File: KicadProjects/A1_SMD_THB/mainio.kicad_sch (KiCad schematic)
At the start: 6 parts, among them J3 PCF, J5 EXF, J6 THO, J7 HE, J8 BL_PROBE, J9 BL_SERVO

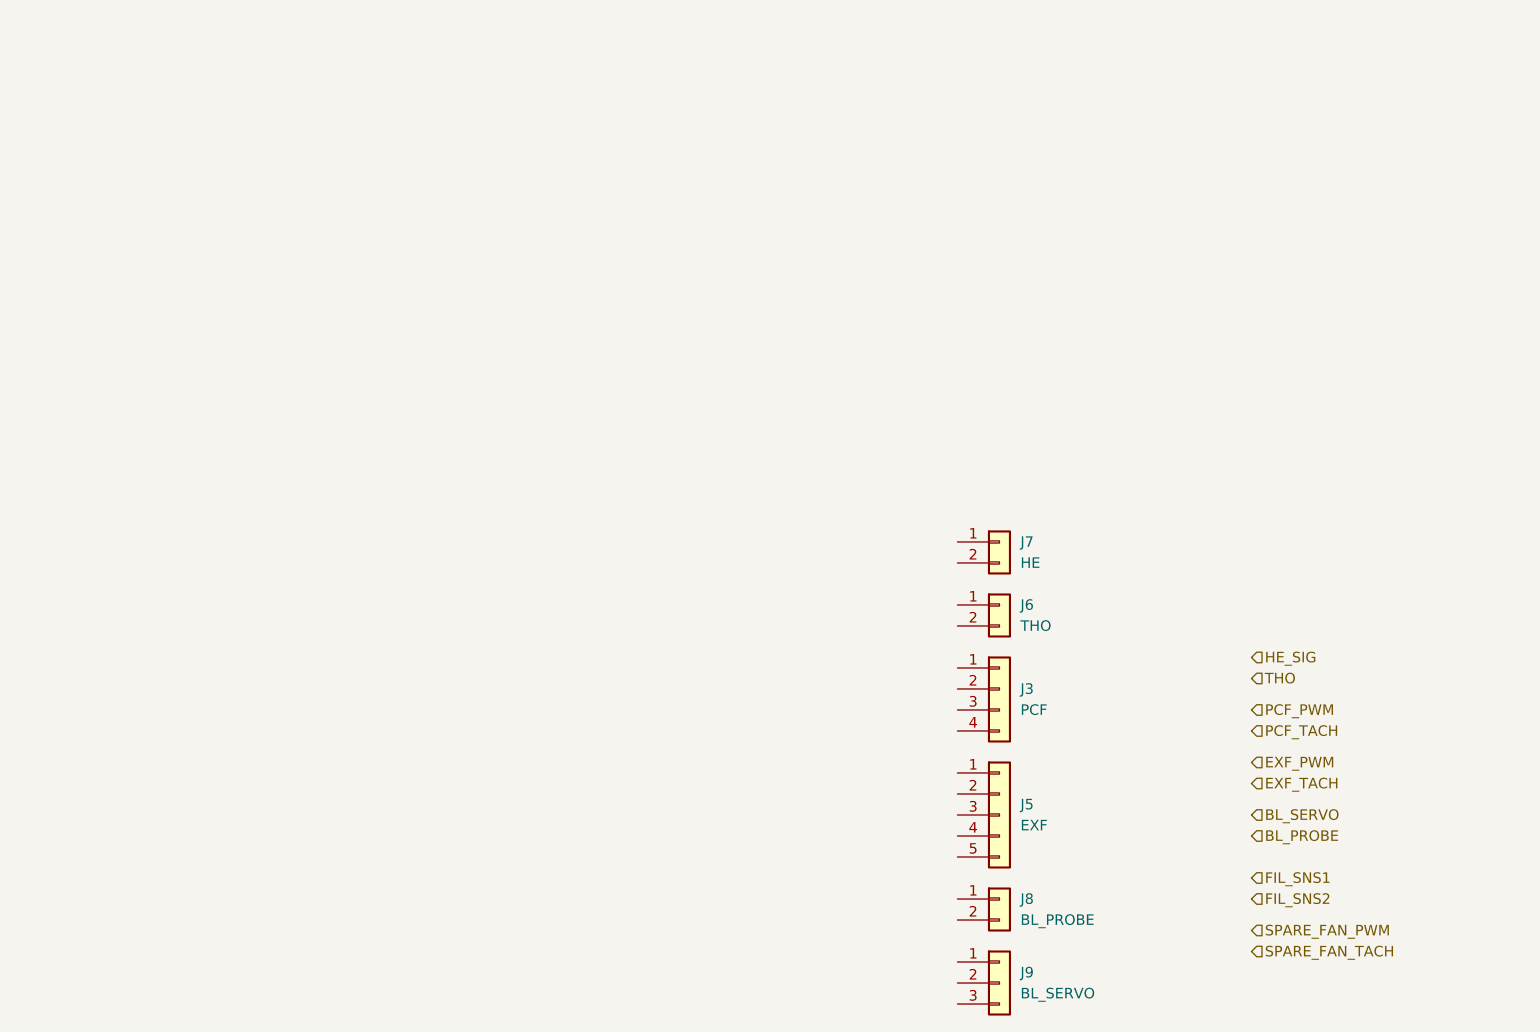
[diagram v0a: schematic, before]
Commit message: e
e
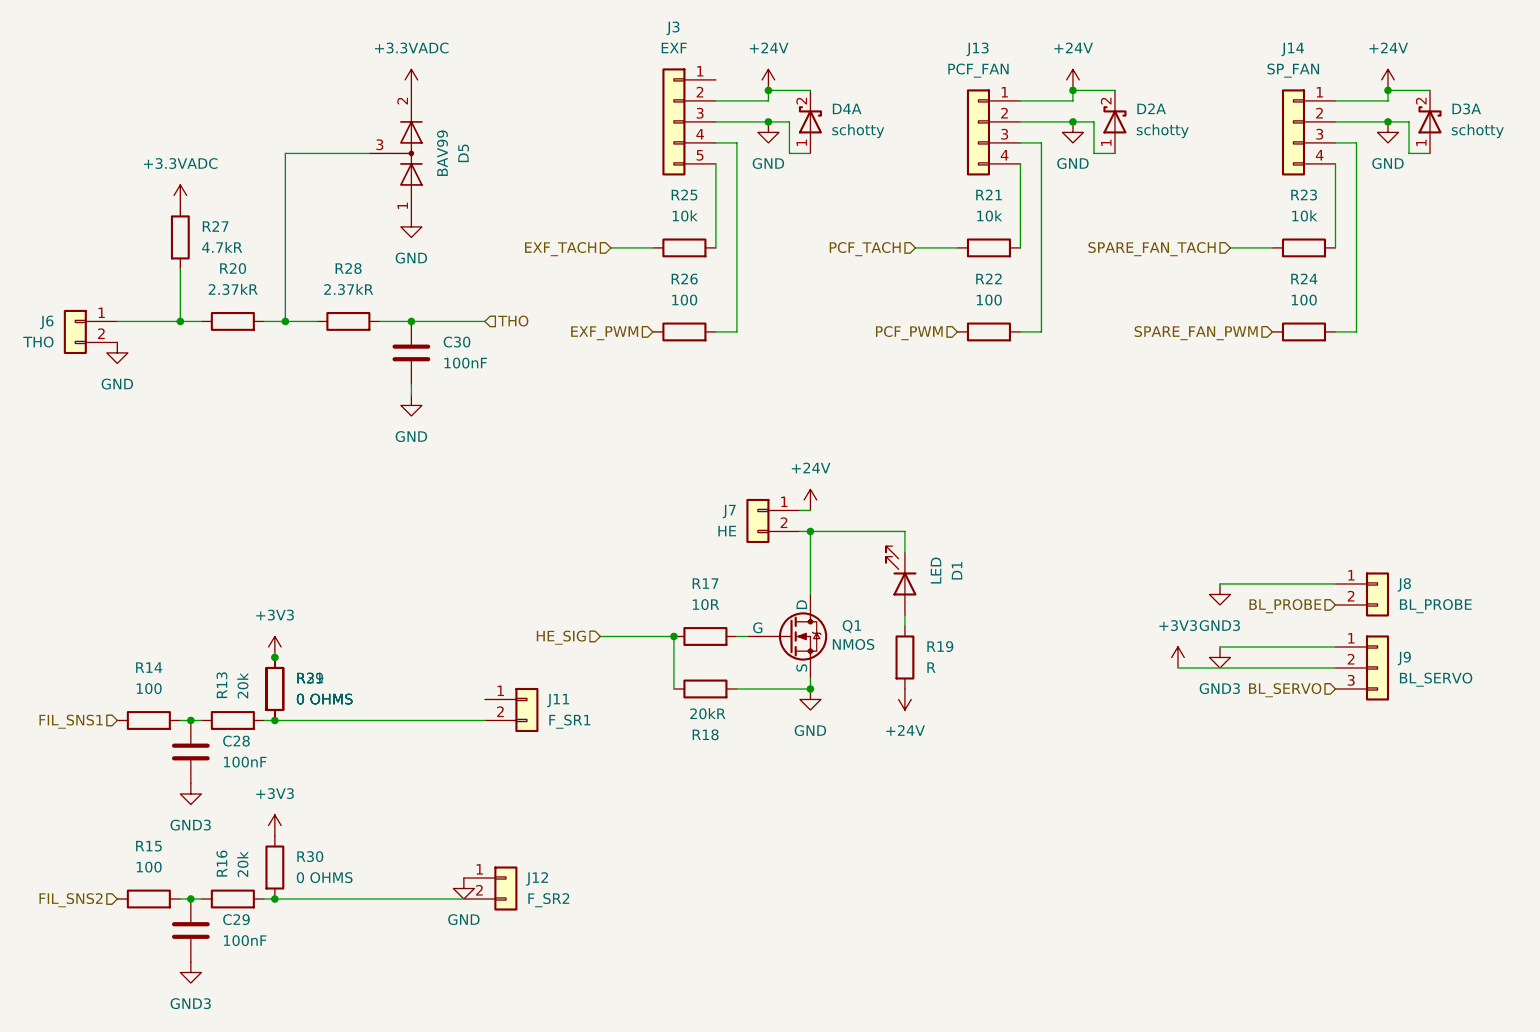
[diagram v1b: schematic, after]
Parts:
- removed J3: PCF, Connector_JST:JST_XH_B4B-XH-A_1x04_P2.50mm_Vertical, symbol Connector_Generic:Conn_01x04
- removed J5: EXF, Connector_JST:JST_XH_B5B-XH-A_1x05_P2.50mm_Vertical, symbol Connector_Generic:Conn_01x05
- added C28, C29, C30: 100nF, Capacitor_SMD:C_0402_1005Metric, symbol Device:C
- added D1: LED, symbol Device:LED
- added D2, D3, D4: schotty, symbol Device:D_Schottky_Dual_CommonAnode_AKK_Split
- added D5: BAV99, Package_TO_SOT_SMD:SOT-23, symbol Diode:BAV99
- added J11: F_SR1, symbol Connector_Generic:Conn_01x02
- added J12: F_SR2, symbol Connector_Generic:Conn_01x02
- added J13: PCF_FAN, symbol Connector_Generic:Conn_01x04
- added J14: SP_FAN, symbol Connector_Generic:Conn_01x04
- added J3: EXF, symbol Connector_Generic:Conn_01x05
- added Q1: NMOS, symbol Simulation_SPICE:NMOS
- added R13, R16: 20k, symbol Device:R
- added R14, R15, R22, R24, R26: 100, symbol Device:R
- added R17: 10R, symbol Device:R
- added R18: 20kR, symbol Device:R
- added R19: R, symbol Device:R
- added R20, R28: 2.37kR, symbol Device:R
- added R21, R23, R25: 10k, symbol Device:R
- added R27: 4.7kR, symbol Device:R
- added R29, R30, R31: 0 OHMS, symbol Device:R
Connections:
- net BL_PROBE: now also J8.2 (Pin_2)
- net BL_SERVO: now also J9.3 (Pin_3)
- net EXF_PWM: now also R26.1
- net EXF_TACH: now also R25.1
- net FIL_SNS1: now also R14.1
- net FIL_SNS2: now also R15.1
- net HE_SIG: now also R17.1, R18.1
- net PCF_PWM: now also R22.1
- net PCF_TACH: now also R21.1
- net SPARE_FAN_PWM: now also R24.1
- net SPARE_FAN_TACH: now also R23.1
- net THO: now also C30.1, R28.2
- net at J6.1 (Pin_1): now also R20.1, R27.2
- net GND: now reaches J6.2 (Pin_2)
- net GND: now also C30.2, D2.1 (A), D3.1 (A), D4.1 (A), D5.1 (K), J12.1 (Pin_1), J13.2 (Pin_2), J14.2 (Pin_2), J3.3 (Pin_3), Q1.3 (S), R18.2
- net GND3: now reaches J9.1 (Pin_1)
- net GND3: now also J8.1 (Pin_1), C28.2, C29.2
- net +3V3: now reaches J9.2 (Pin_2)
- net +3V3: now also R29.1, R30.1, R31.1
- net +24V: now reaches J7.1 (Pin_1)
- net +24V: now also D2.2 (K), D3.2 (K), D4.2 (K), J13.1 (Pin_1), J14.1 (Pin_1), J3.2 (Pin_2), R19.2
- net at J7.2 (Pin_2): now also D1.1 (K), Q1.1 (D)
- new net: J14.3 (Pin_3), R24.2
- new net: J14.4 (Pin_4), R23.2
- new net: C28.1, R13.1, R14.2
- new net: D1.2 (A), R19.1
- new net: J11.2 (Pin_2), R13.2, R29.2, R31.2
- new net: Q1.2 (G), R17.2
- new net: D5.3 (K), R20.2, R28.1
- new net: J13.3 (Pin_3), R22.2
- new net: J3.4 (Pin_4), R26.2
- new net: J13.4 (Pin_4), R21.2
- new net: J3.5 (Pin_5), R25.2
- new net: C29.1, R15.2, R16.1
- new net: J12.2 (Pin_2), R16.2, R30.2
- new net +3.3VADC: D5.2 (A), R27.1
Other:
- moved on the sheet: J6, J7, J8, J9
